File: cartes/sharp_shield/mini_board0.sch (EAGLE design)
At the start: 18 parts, among them Q1 16MHz, U1 MCP2551

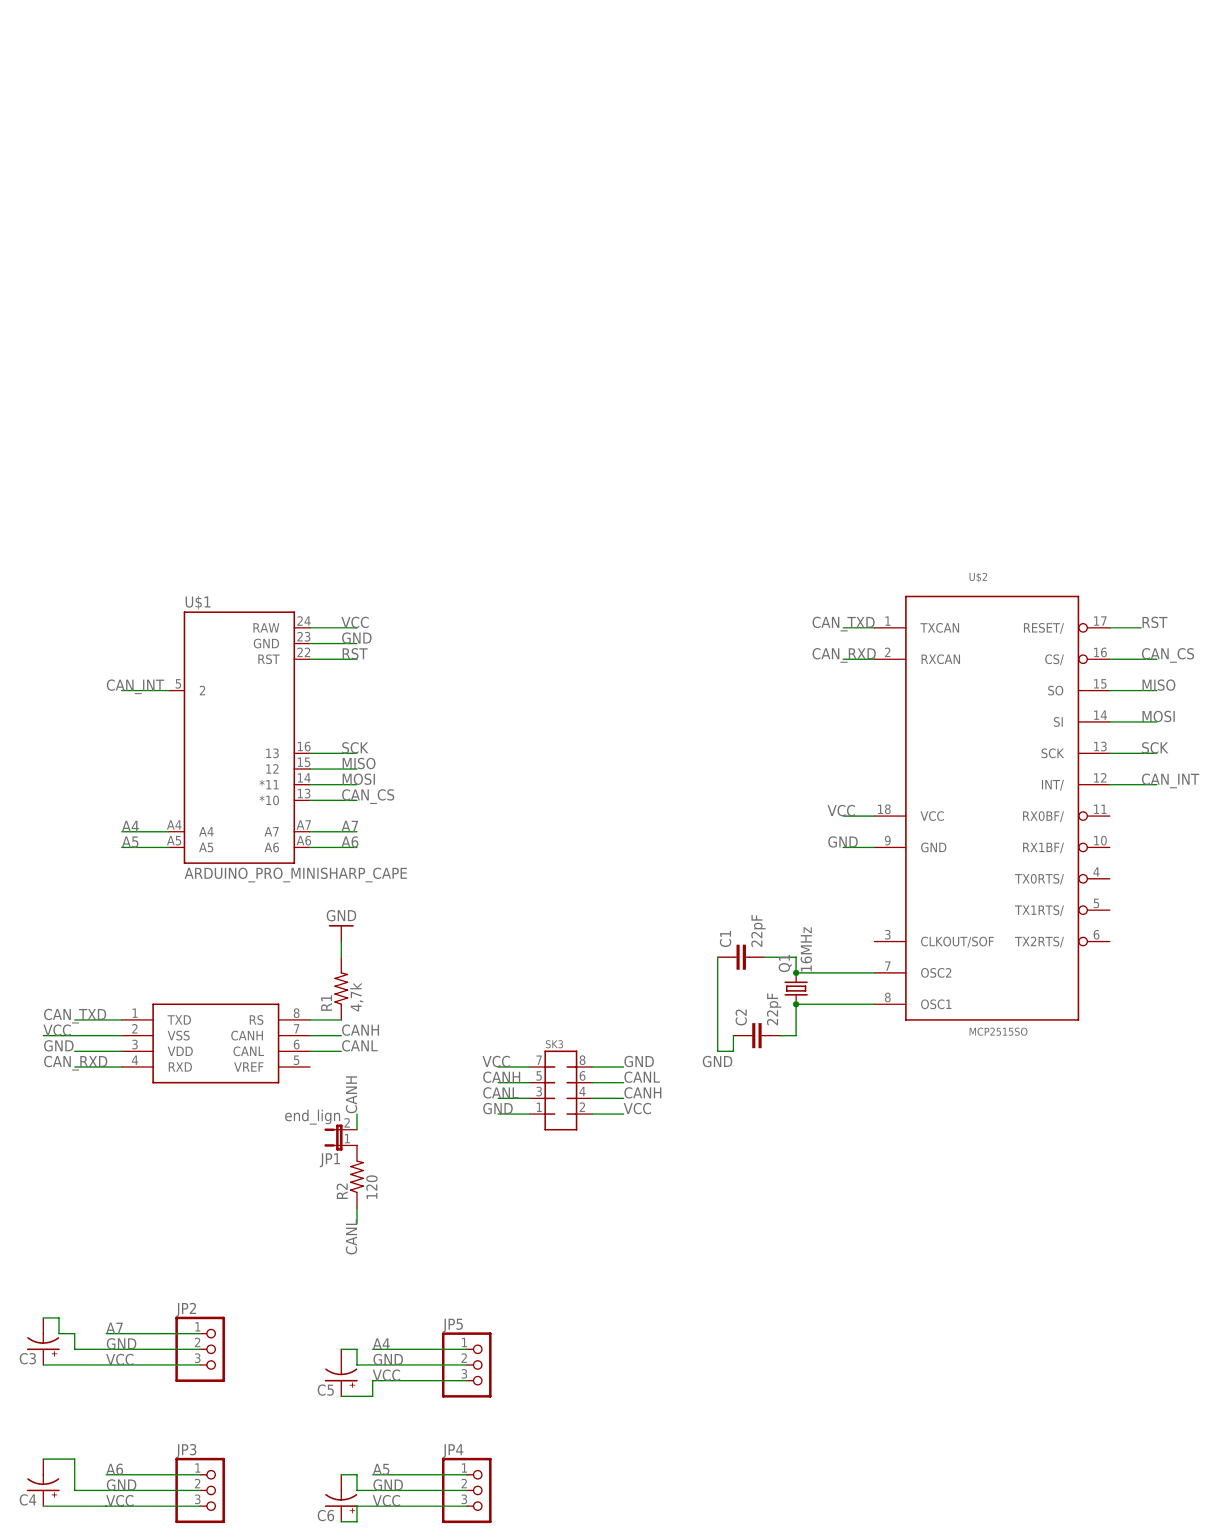
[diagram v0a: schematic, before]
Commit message: divers
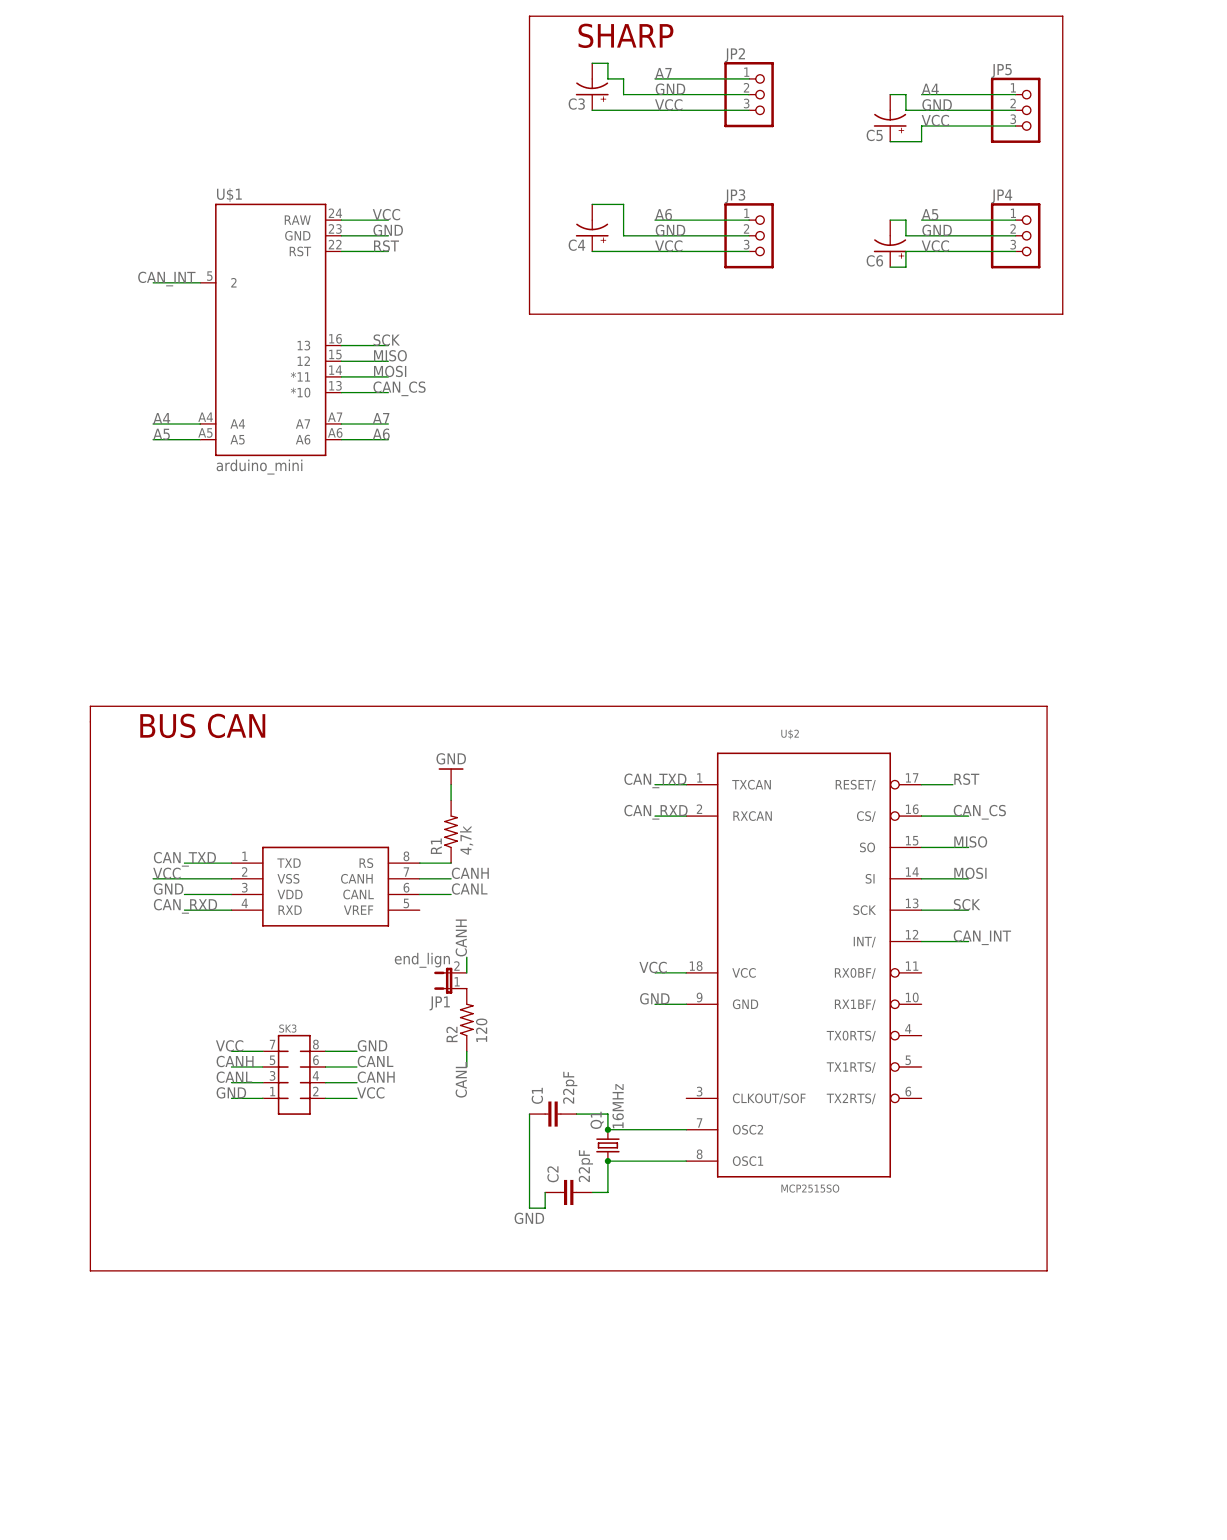
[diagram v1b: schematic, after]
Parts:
- U$1: value ARDUINO_PRO_MINISHARP_CAPE -> arduino_mini
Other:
- note added: "BUS CAN"
- note added: "SHARP"
- moved on the sheet: C1, C2, C3, C4, C5, C6, JP1, JP2, JP3, JP4, JP5, Q1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
